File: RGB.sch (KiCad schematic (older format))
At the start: 4 parts

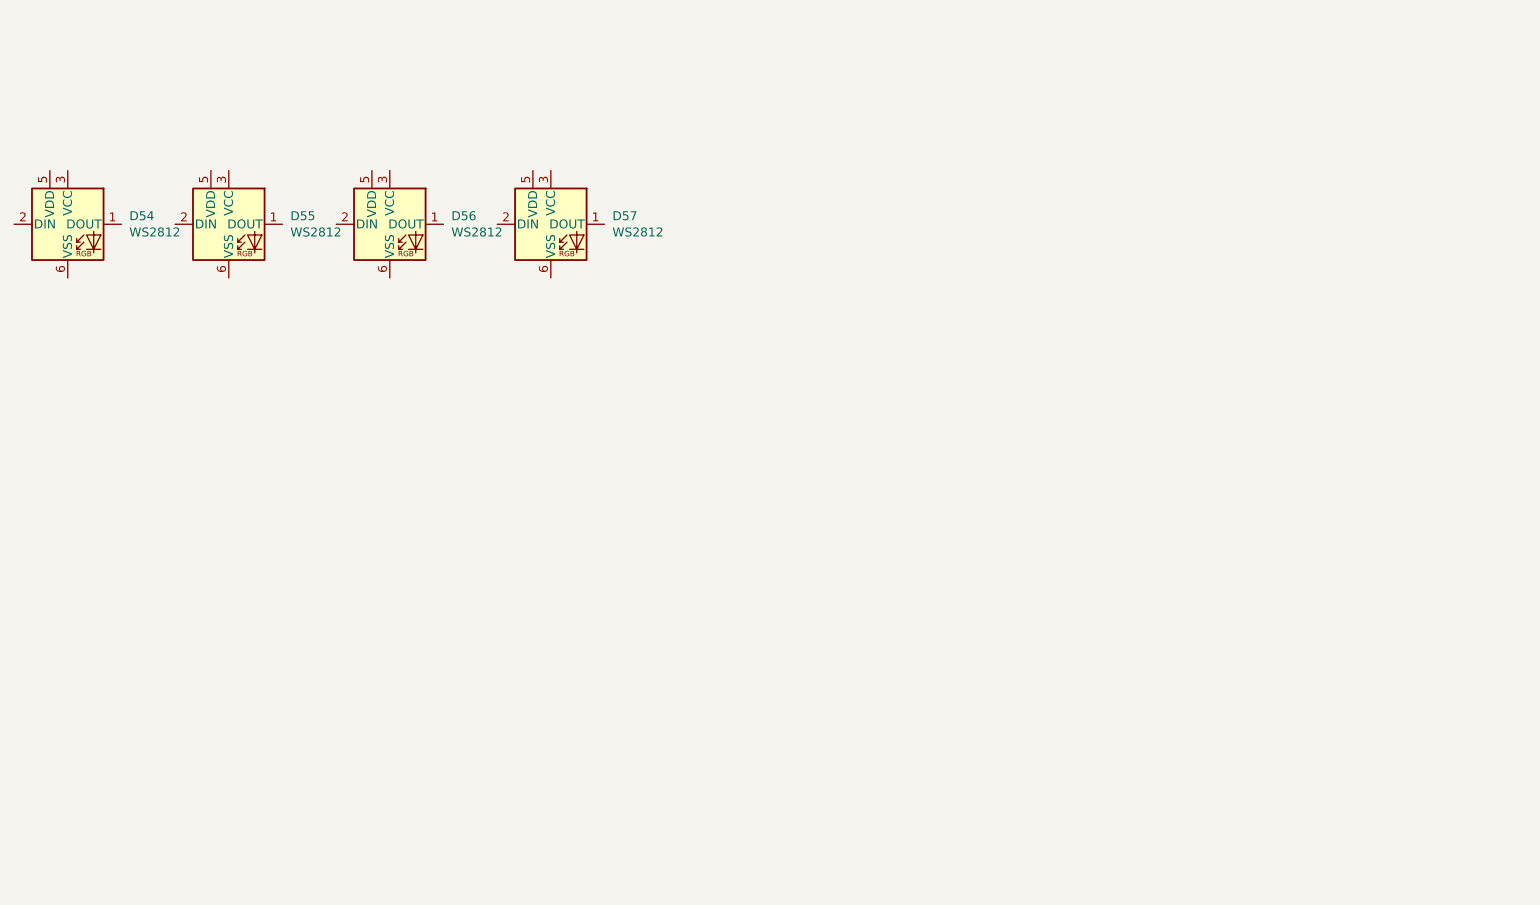
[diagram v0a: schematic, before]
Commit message: Position switch matrix
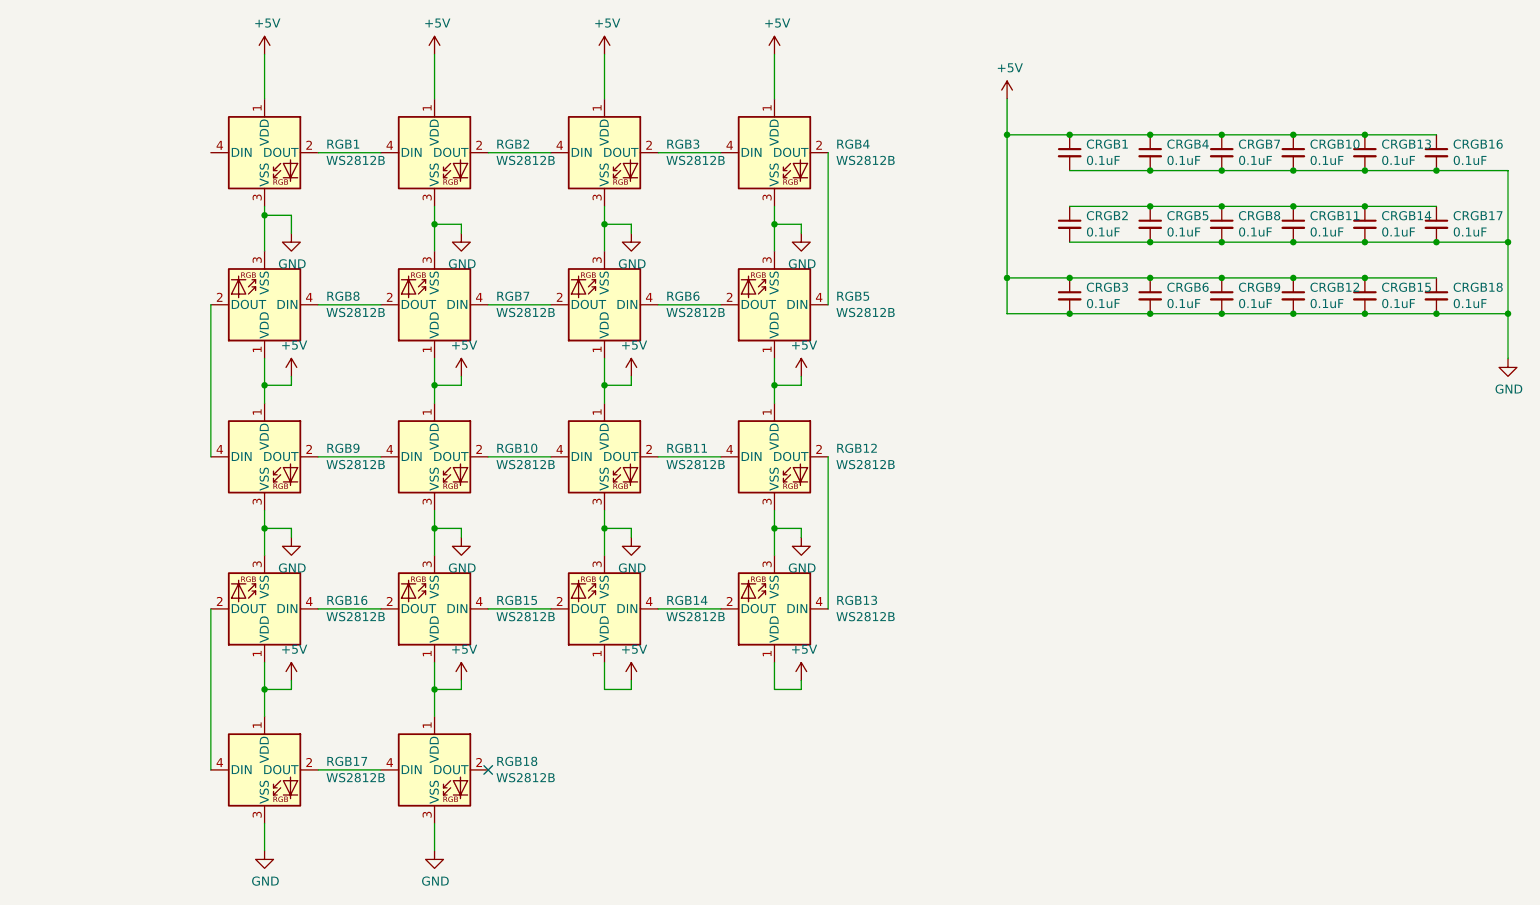
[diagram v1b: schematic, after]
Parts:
- removed D54, D55, D56, D57: WS2812, LED_SMD:LED_WS2812_PLCC6_5.0x5.0mm_P1.6mm, symbol LED:WS2812
- added CRGB1, CRGB10, CRGB11, CRGB12, CRGB13, CRGB14, CRGB15, CRGB16, CRGB17, CRGB18, CRGB2, CRGB3, CRGB4, CRGB5, CRGB6, CRGB7, CRGB8, CRGB9: 0.1uF, Capacitor_SMD:C_0805_2012Metric_Pad1.15x1.40mm_HandSolder, symbol Device:C_Small
- added RGB1, RGB10, RGB11, RGB12, RGB13, RGB14, RGB15, RGB16, RGB17, RGB18, RGB2, RGB3, RGB4, RGB5, RGB6, RGB7, RGB8, RGB9: WS2812B, LED_SMD:LED_WS2812B_PLCC4_5.0x5.0mm_P3.2mm, symbol LED:WS2812B
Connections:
- new net: RGB1.2 (DOUT), RGB2.4 (DIN)
- new net: RGB2.2 (DOUT), RGB3.4 (DIN)
- new net: RGB8.2 (DOUT), RGB9.4 (DIN)
- new net: RGB7.2 (DOUT), RGB8.4 (DIN)
- new net: RGB6.2 (DOUT), RGB7.4 (DIN)
- new net: RGB10.4 (DIN), RGB9.2 (DOUT)
- new net: RGB10.2 (DOUT), RGB11.4 (DIN)
- new net: RGB16.2 (DOUT), RGB17.4 (DIN)
- new net: RGB15.2 (DOUT), RGB16.4 (DIN)
- new net: RGB14.2 (DOUT), RGB15.4 (DIN)
- new net: RGB3.2 (DOUT), RGB4.4 (DIN)
- new net: RGB4.2 (DOUT), RGB5.4 (DIN)
- new net: RGB5.2 (DOUT), RGB6.4 (DIN)
- new net: RGB11.2 (DOUT), RGB12.4 (DIN)
- new net: RGB12.2 (DOUT), RGB13.4 (DIN)
- new net: RGB13.2 (DOUT), RGB14.4 (DIN)
- new net: RGB17.2 (DOUT), RGB18.4 (DIN)
- new net: CRGB11.1, CRGB14.1, CRGB17.1, CRGB2.1, CRGB5.1, CRGB8.1
- new net +5V: CRGB1.1, CRGB1.2, CRGB10.1, CRGB10.2, CRGB11.2, CRGB12.1, CRGB12.2, CRGB13.1, CRGB13.2, CRGB14.2, CRGB15.1, CRGB15.2, CRGB16.1, CRGB16.2, CRGB17.2, CRGB18.1, CRGB18.2, CRGB2.2, CRGB3.1, CRGB3.2, CRGB4.1, CRGB4.2, CRGB5.2, CRGB6.1, CRGB6.2, CRGB7.1, CRGB7.2, CRGB8.2, CRGB9.1, CRGB9.2, RGB1.1 (VDD), RGB1.3 (VSS), RGB10.1 (VDD), RGB10.3 (VSS), RGB11.1 (VDD), RGB11.3 (VSS), RGB12.1 (VDD), RGB12.3 (VSS), RGB13.1 (VDD), RGB13.3 (VSS), RGB14.1 (VDD), RGB14.3 (VSS), RGB15.1 (VDD), RGB15.3 (VSS), RGB16.1 (VDD), RGB16.3 (VSS), RGB17.1 (VDD), RGB17.3 (VSS), RGB18.1 (VDD), RGB18.3 (VSS), RGB2.1 (VDD), RGB2.3 (VSS), RGB3.1 (VDD), RGB3.3 (VSS), RGB4.1 (VDD), RGB4.3 (VSS), RGB5.1 (VDD), RGB5.3 (VSS), RGB6.1 (VDD), RGB6.3 (VSS), RGB7.1 (VDD), RGB7.3 (VSS), RGB8.1 (VDD), RGB8.3 (VSS), RGB9.1 (VDD), RGB9.3 (VSS)
- no-connect marks 0 -> 1
